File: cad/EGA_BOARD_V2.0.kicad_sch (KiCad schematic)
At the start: 14 parts, among them SW1 SWITCH (B3F-1020), SW2 SWITCH (B3F-1020), SW3 SWITCH (B3F-1020)

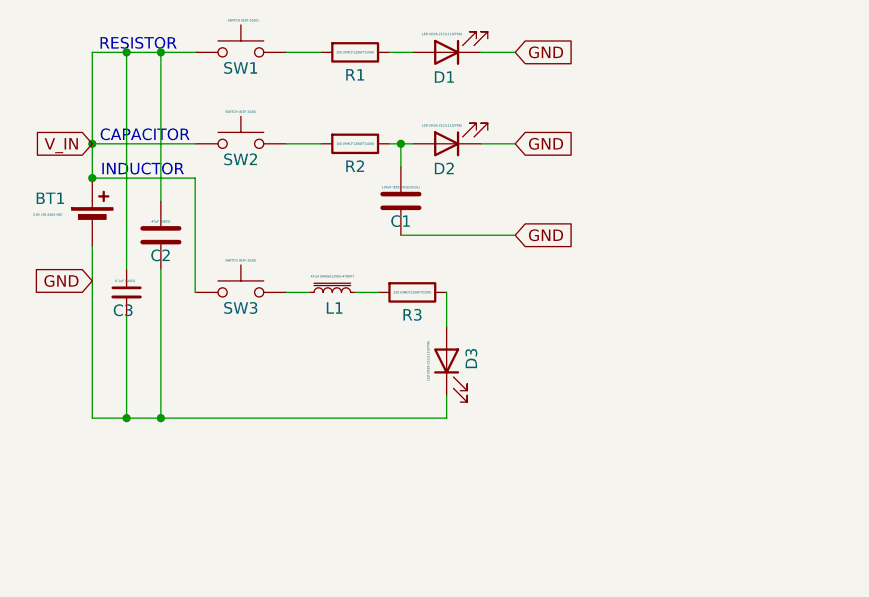
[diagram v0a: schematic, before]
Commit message: EDITED BOARD
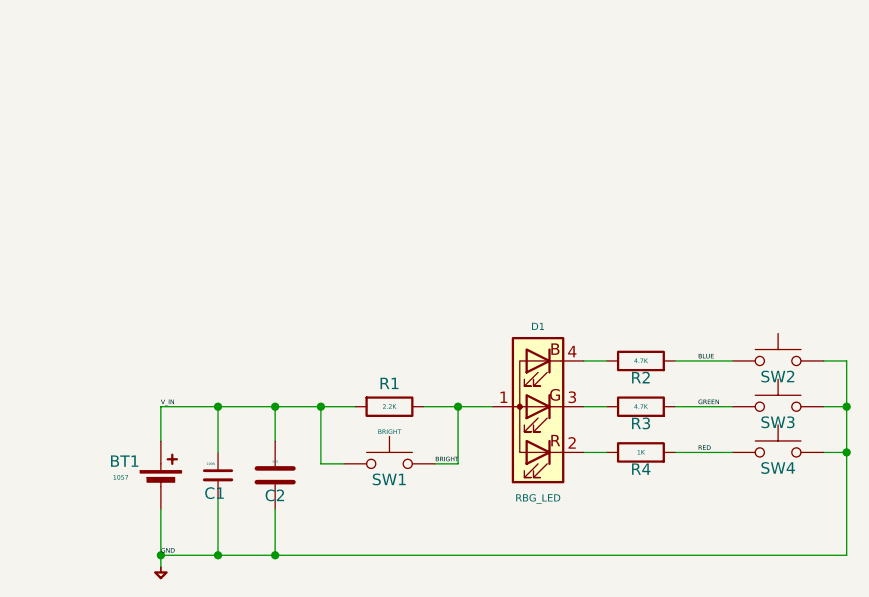
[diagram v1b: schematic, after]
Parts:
- removed C1: 100uF (EEE-FH1E101XL), Capacitor_SMD:C_Elec_5x5.8, symbol Device:C
- removed C3: 0.1uF (0603), Capacitor_SMD:C_0603_1608Metric, symbol Device:C_Small
- removed D1, D2, D3: LED (IR26-21C/L110/TR8), LED_SMD:LED_1206_3216Metric, symbol LED:IR26-21C_L110_TR8
- removed L1: 47uH (MWSA1206S-470MT), Inductor_SMD:L_Sunlord_MWSA1206S-3R3, symbol Device:L_Iron_Small
- added C1: 100N, CAPS:C_0603_1608Metric, symbol Device:C_Small
- added D1: RBG_LED, LED:LED_Cree-PLCC4_3.2x2.8mm_CCW, symbol LED (X3):CLV1L-FKB
- added R4: 1K, CAPS:C_0603_1608Metric, symbol Device:R
- added SW4: SWITCH (B3F-1020), BUTTON_SWITCH:SW_TH_Tactile_Omron_B3F-102x, symbol Switch:SW_Push
- BT1: value 3.0V (36-2462-ND) -> 1057; footprint Battery:BatteryHolder_Keystone_2462_2xAA -> SIG_PLAYGND:BAT_1057
- C2: value 47uF (0805) -> 10U; footprint Capacitor_SMD:C_0805_2012Metric -> CAPS:C_0805_2012Metric
- R1: value 100 (RMCF1206FT100R) -> 2.2K; footprint Resistor_SMD:R_1206_3216Metric -> CAPS:C_0603_1608Metric
- R2: value 100 (RMCF1206FT100R) -> 4.7K; footprint Resistor_SMD:R_1206_3216Metric -> CAPS:C_0603_1608Metric
- R3: value 220 (RMCF1206FT220R) -> 4.7K; footprint Resistor_SMD:R_1206_3216Metric -> CAPS:C_0603_1608Metric
- SW1: value SWITCH (B3F-1020) -> BRIGHT; footprint Button_Switch_THT:SW_TH_Tactile_Omron_B3F-102x -> BUTTON_SWITCH:SW_SPST_Omron_B3FS-100xP
- SW2, SW3: footprint Button_Switch_THT:SW_TH_Tactile_Omron_B3F-102x -> BUTTON_SWITCH:SW_TH_Tactile_Omron_B3F-102x
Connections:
- net GND: now also SW2.2, SW3.2, C1.2, SW4.2
- net V_IN: now also R1.2, C1.1; no longer SW2.1, SW3.1
- net GREEN: now reaches R3.2
- net GREEN: now also SW3.1
- net at R2.1: now also D1.4 (BK)
- net at R3.1: now also D1.3 (GK)
- net BRIGHT: now reaches R1.1
- net BRIGHT: now also SW1.2, D1.1 (A)
- net BLUE: now reaches R2.2
- net BLUE: now also SW2.1; no longer SW2.2
- new net: D1.2 (RK), R4.1
- new net RED: R4.2, SW4.1
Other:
- note removed: "CAPACITOR"
- note removed: "INDUCTOR"
- note removed: "RESISTOR"
